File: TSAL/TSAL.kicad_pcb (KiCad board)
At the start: 2 copper layers, 42 parts, among them J1 Conn_02x03_Counter_Clockwise, J2 Conn_01x02, J4 Conn_02x01, U1 LM358, U2 4002, U3 74HC00, U4 4N35, U5 74HC21, U6 74HC7014, U7 LM7805_TO220, U8 LM339, U9 LM339

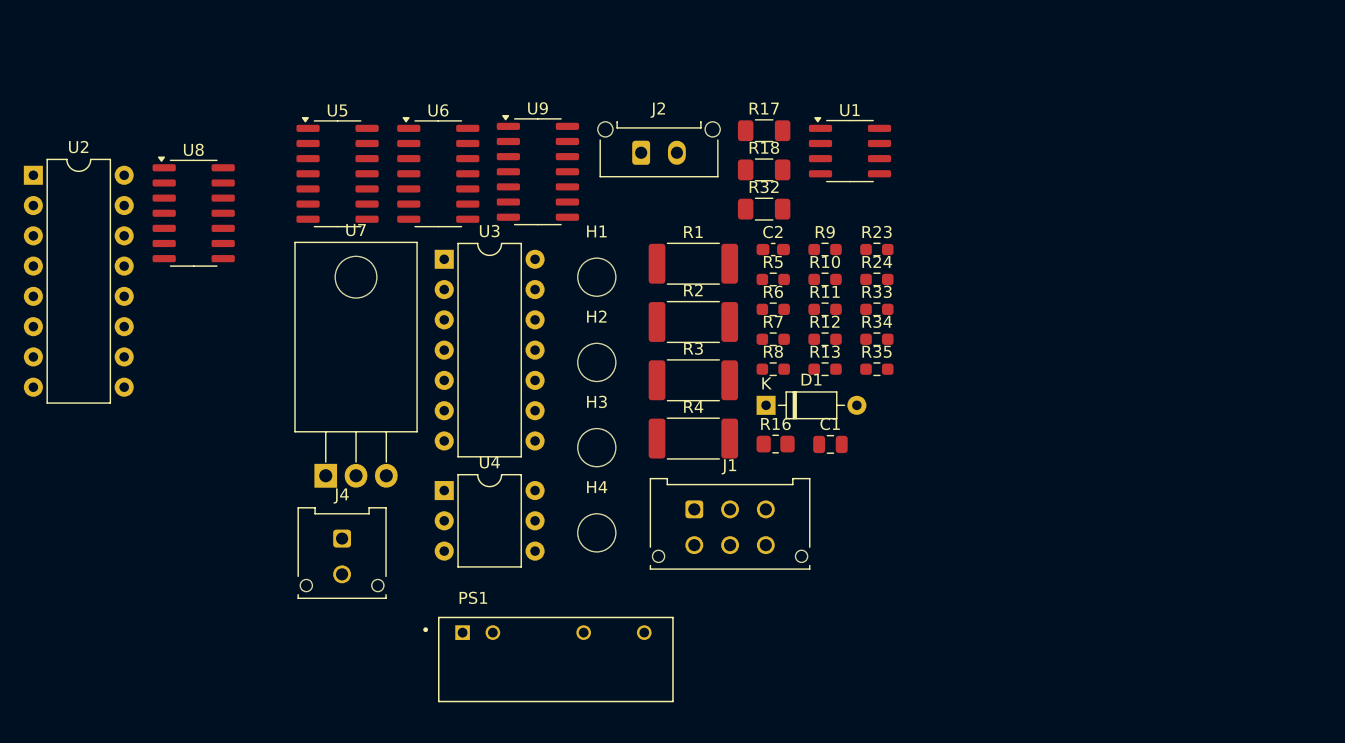
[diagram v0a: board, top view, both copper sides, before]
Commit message: CREATE TSAL PCBs
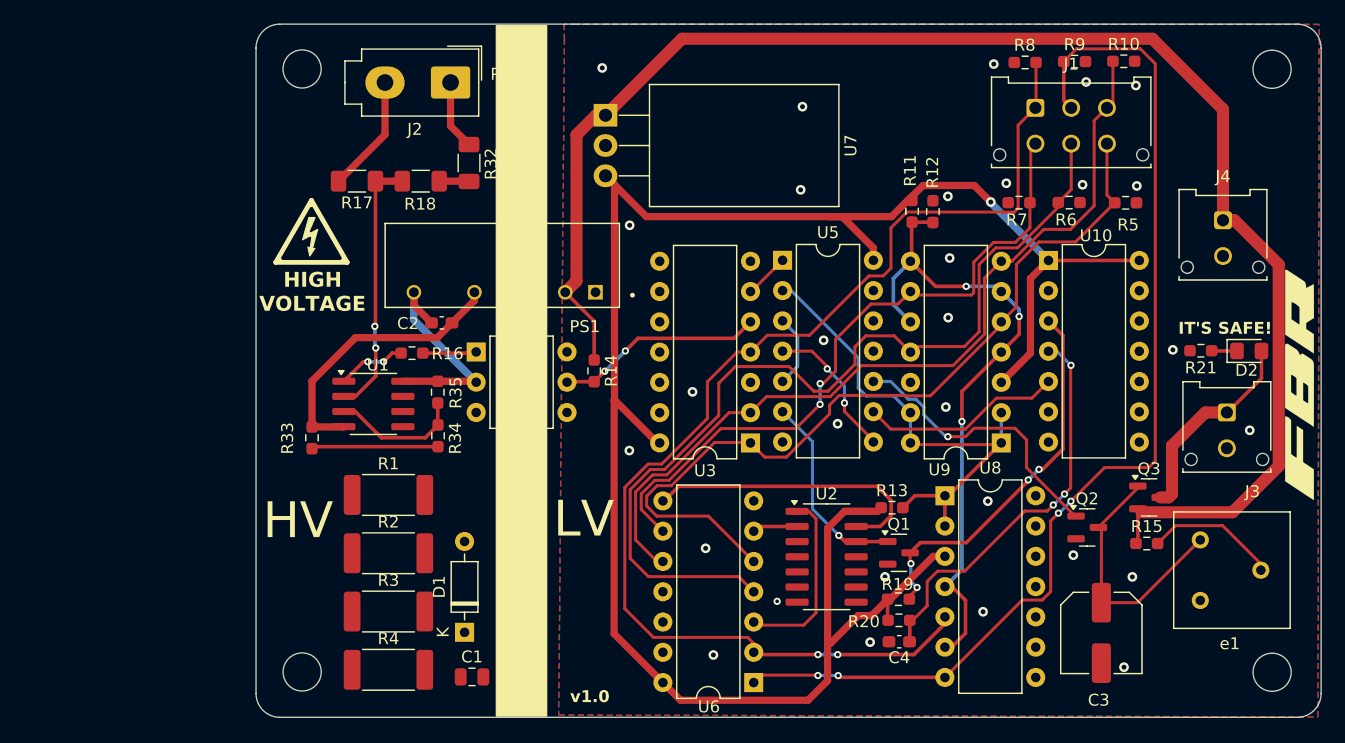
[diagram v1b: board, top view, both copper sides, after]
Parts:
- removed R23: 22K, Resistor_SMD:R_0603_1608Metric_Pad0.98x0.95mm_HandSolder
- removed R24: 33K, Resistor_SMD:R_0603_1608Metric_Pad0.98x0.95mm_HandSolder
- added C3: 100uF, Capacitor_SMD:C_Elec_6.3x7.7, F.Cu at (129.4, 81.9)
- added C4: 0.1uF, Capacitor_SMD:C_0603_1608Metric_Pad1.08x0.95mm_HandSolder, F.Cu at (112.4, 82.6)
- added D2: GRN, LED_SMD:LED_0805_2012Metric_Pad1.15x1.40mm_HandSolder, F.Cu at (141.8, 58.2)
- added G***: LOGO, LOGO, F.Cu at (146.0, 61.2)
- added J3: Conn_02x01, Connector_Molex:Molex_Micro-Fit_3.0_43045-0212_2x01_P3.00mm_Vertical, F.Cu at (139.9, 63.4)
- added Q1: BSS138, Package_TO_SOT_SMD:SOT-23, F.Cu at (112.4, 75.2)
- added Q2: BSS138, Package_TO_SOT_SMD:SOT-23, F.Cu at (128.2, 73.0)
- added Q3: AO3401A, Package_TO_SOT_SMD:SOT-23, F.Cu at (133.4, 70.5)
- added R14: 12K, Resistor_SMD:R_0603_1608Metric_Pad0.98x0.95mm_HandSolder, F.Cu at (86.8, 59.9)
- added R15: 7.5K, Resistor_SMD:R_0603_1608Metric_Pad0.98x0.95mm_HandSolder, F.Cu at (133.2, 74.4)
- added R19: 10K, Resistor_SMD:R_0603_1608Metric_Pad0.98x0.95mm_HandSolder, F.Cu at (112.4, 79.1)
- added R20: 10K, Resistor_SMD:R_0603_1608Metric_Pad0.98x0.95mm_HandSolder, F.Cu at (112.4, 80.8)
- added R21: 2k2, Resistor_SMD:R_0603_1608Metric_Pad0.98x0.95mm_HandSolder, F.Cu at (137.7, 58.2)
- added REF**: Symbol_HighVoltage_Triangle_6x6mm_Copper, Symbol:Symbol_HighVoltage_Triangle_6x6mm_Copper, F.Cu at (63.1, 48.2)
- added U10: 74HC74, Package_DIP:DIP-14_W7.62mm, F.Cu at (124.9, 50.6)
- added e1: R_Potentiometer_Trim, Potentiometer_THT:Potentiometer_Bourns_3386F_Vertical, F.Cu at (137.7, 79.2)
- J2: footprint Connector_Molex:Molex_Micro-Fit_3.0_43650-0215_1x02_P3.00mm_Vertical -> Connector_Molex:Molex_Mini-Fit_Jr_5566-02A_2x01_P4.20mm_Vertical
- R13: value 12K -> 10K
- R16: value 1K -> 500; footprint Resistor_SMD:R_0805_2012Metric_Pad1.20x1.40mm_HandSolder -> Resistor_SMD:R_0603_1608Metric_Pad0.98x0.95mm_HandSolder
- U2: value 4002 -> 74HC27; footprint Package_DIP:DIP-16_W7.62mm -> Package_SO:SOIC-14_3.9x8.7mm_P1.27mm
- U3: value 74HC00 -> 74HC20
- U5: value 74HC21 -> 74HC08; footprint Package_SO:SOIC-14_3.9x8.7mm_P1.27mm -> Package_DIP:DIP-14_W7.62mm
- U6: value 74HC7014 -> 74HC86; footprint Package_SO:SOIC-14_3.9x8.7mm_P1.27mm -> Package_DIP:DIP-14_W7.62mm
- U8, U9: footprint Package_SO:SOIC-14_3.9x8.7mm_P1.27mm -> Package_DIP:DIP-14_W7.62mm
- moved J4 78.6 mm to (139.6, 47.3)
- moved U2 73.8 mm to (106.3, 75.5)
- moved U8 67.3 mm to (116.2, 70.4)
- moved H3 64.9 mm to (143.7, 34.6)
- moved H4 57.8 mm to (143.7, 85.2)
- moved U6 50.2 mm to (100.2, 86.1), turned to 180 degrees
- moved R33 48.6 mm to (63.1, 65.5), turned to -90 degrees
- moved U1 45.3 mm to (68.3, 62.7)
- moved U9 45.0 mm to (121.0, 66.0), turned to 180 degrees
- moved J1 44.2 mm to (123.8, 37.8)
- moved U7 38.3 mm to (87.8, 38.5), turned to -90 degrees
- moved U5 38.0 mm to (102.6, 50.6)
- moved R34 37.7 mm to (73.7, 65.4), turned to 90 degrees
- moved R35 36.9 mm to (73.7, 61.7), turned to 90 degrees
- moved H2 35.9 mm to (62.3, 85.2)
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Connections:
- J1 pad 1: /AIR+ -> /Precharge
- J1 pad 2: /AIR+_Int -> /PreCh_Int
- J1 pad 3: /AIR-_Int -> /AIR-
- J1 pad 4: /AIR- -> /AIR-_Int
- J1 pad 5: /PreCh_Int -> /AIR+_Int
- J1 pad 6: /Precharge -> /AIR+
- R13 pad 1: GLV+ -> /5V
- U2 pad 1: /GRN_OK -> Net-(U2-Pad1)
- U2 pad 12: unconnected-(U2-Pad12) -> /PLUASBL_CHK
- U2 pad 13: unconnected-(U2-Pad13) -> Net-(U2-Pad13)_1
- U2 pad 2: /AIR+_TSAL -> Net-(U2-Pad2)
- U2 pad 3: /AIR-_TSAL -> (no net)
- U2 pad 4: /Precharge_TSAL -> (no net)
- U2 pad 5: /VHI<60V -> (no net)
- U3 pad 1: /PreCh_Int -> /AIR+
- U3 pad 10: /AIR- -> unconnected-(U3-Pad10)
- U3 pad 11: unconnected-(U3-Pad11) -> (no net)
- U3 pad 2: /Precharge -> /AIR-
- U3 pad 3: unconnected-(U3-Pad3) -> (no net)
- U3 pad 4: /AIR+_Int -> /Precharge
- U3 pad 5: /AIR+ -> /~{VHI<60V}
- U3 pad 6: unconnected-(U3-Pad6) -> /GRN_OK
- U3 pad 8: (no net) -> unconnected-(U3-Pad8)
- U3 pad 9: /AIR-_Int -> unconnected-(U3-Pad9)
- U4 pad 4: Net-(R24-Pad1) -> GLV-
- U4 pad 5: GLV+ -> /~{VHI<60V}
- U5 pad 1: (no net) -> /GRN_OK
- U5 pad 10: (no net) -> Net-(Q2-G)
- U5 pad 11: (no net) -> unconnected-(U5-Pad11)
- U5 pad 12: (no net) -> unconnected-(U5-Pad12)
- U5 pad 13: (no net) -> unconnected-(U5-Pad13)
- U5 pad 2: (no net) -> /SCS_Compliance
- U5 pad 3: (no net) -> Net-(U5-Pad3)
- U5 pad 4: (no net) -> /GRN_LIGHT
- U5 pad 5: (no net) -> Net-(U5-Pad3)
- U5 pad 6: (no net) -> /PLUASBL_CHK
- U5 pad 8: (no net) -> /GRN_LIGHT
- U5 pad 9: (no net) -> Net-(U10A-Q)
- U6 pad 1: (no net) -> /PreCh_Int
- U6 pad 10: (no net) -> /AIR-
- U6 pad 11: (no net) -> unconnected-(U6-Pad11)
- U6 pad 12: (no net) -> unconnected-(U6-Pad12)
- U6 pad 13: (no net) -> unconnected-(U6-Pad13)
- U6 pad 2: (no net) -> /Precharge
- U6 pad 3: (no net) -> Net-(U2-Pad1)
- U6 pad 4: (no net) -> /AIR+_Int
- U6 pad 5: (no net) -> /AIR+
- U6 pad 6: (no net) -> Net-(U2-Pad2)
- U6 pad 8: (no net) -> Net-(U2-Pad13)_1
- U6 pad 9: (no net) -> /AIR-_Int
- U8 pad 3: GLV+ -> /5V
- U9 pad 3: GLV+ -> /5V
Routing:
- net /5V: track 0.00 -> 165.4 mm, vias 0 -> 1
- net GLV+: track 0.00 -> 129.3 mm
- net /Precharge: track 0.00 -> 100.1 mm, vias 0 -> 2
- net /PreCh_Int: track 0.00 -> 92.3 mm, vias 0 -> 4
- net /AIR+_Int: track 0.00 -> 77.4 mm
- net /AIR-: track 0.00 -> 71.0 mm
- net /AIR+: track 0.00 -> 70.2 mm
- net /AIR-_Int: track 0.00 -> 57.7 mm, vias 0 -> 2
- net /.25V: track 0.00 -> 54.7 mm, vias 0 -> 3
- net /SCS_Compliance: track 0.00 -> 43.0 mm
- net Net-(U10A-~{S}): track 0.00 -> 33.8 mm, vias 0 -> 3
- net Net-(Q1-D): track 0.00 -> 32.2 mm, vias 0 -> 4
- net Net-(U2-Pad13)_1: track 0.00 -> 24.7 mm
- net Net-(Q2-G): track 0.00 -> 24.0 mm, vias 0 -> 1
- net /5V+_Iso: track 0.00 -> 23.7 mm
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- added copper zone on B.Cu, net GLV-
- added copper zone on F.Cu, net GLV-
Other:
- board outline added: 89.4 x 58.2 mm
- board text added: "0.2000 mm / 0.2000 mm"
- board text added: "0.3000 mm"
- board text added: "1.6000 mm"
- board text added: "2"
- board text added: "89.3550 mm x 58.1550 mm"
- board text added: "BOARD CHARACTERISTICS"
- board text added: "Board Thickness:"
- board text added: "Board overall dimensions:"
- board text added: "Castellated pads:"
- board text added: "Copper Finish:"
- board text added: "Copper Layer Count:"
- board text added: "Edge card connectors:"
- board text added: "HAL SnPb"
- board text added: "HIGH VOLTAGE"
- board text added: "HV"
- board text added: "IT'S SAFE!"
- board text added: "Impedance Control:"
- board text added: "LV"
- board text added: "Min hole diameter:"
- board text added: "Min track/spacing:"
- board text added: "No"
- board text added: "PS1"
- board text added: "Plated Board Edge:"
- board text added: "v1.0"
